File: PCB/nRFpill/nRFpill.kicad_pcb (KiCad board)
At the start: 2 copper layers, 90.7 x 52.7 mm, 138 parts, among them J1 USB_C_Receptacle_USB2.0, J10 , J11 USB_C_Receptacle_USB2.0, J12 , J13 , J14 , J15 , J16 USB_C_Receptacle_USB2.0, J17 , J18 , J19 , J2 , J20 , J3 , J4 , J5 , J6 USB_C_Receptacle_USB2.0, J7 , J8 , J9 , Q1 AO3407, Q2 AO3407, Q3 AO3407, Q4 AO3407, Q5 AO3407, Q6 AO3407, Q7 AO3407, Q8 AO3407, SW1 RST, SW2 DFU, SW3 RST, SW4 DFU, SW5 RST, SW6 DFU, SW7 RST, SW8 DFU, U1 MIC5219-3.3YM5, U10 USBLC6-2SC6, U11 TP4054, U12 MS88FS3, U13 MIC5219-3.3YM5, U14 USBLC6-2SC6, U15 TP4054, U16 MS88FS3, U2 USBLC6-2SC6, U3 TP4054, U4 MIC5219-3.3YM5, U5 MS88FS3, U6 USBLC6-2SC6, U7 TP4054, U8 MS88FS3, U9 MIC5219-3.3YM5

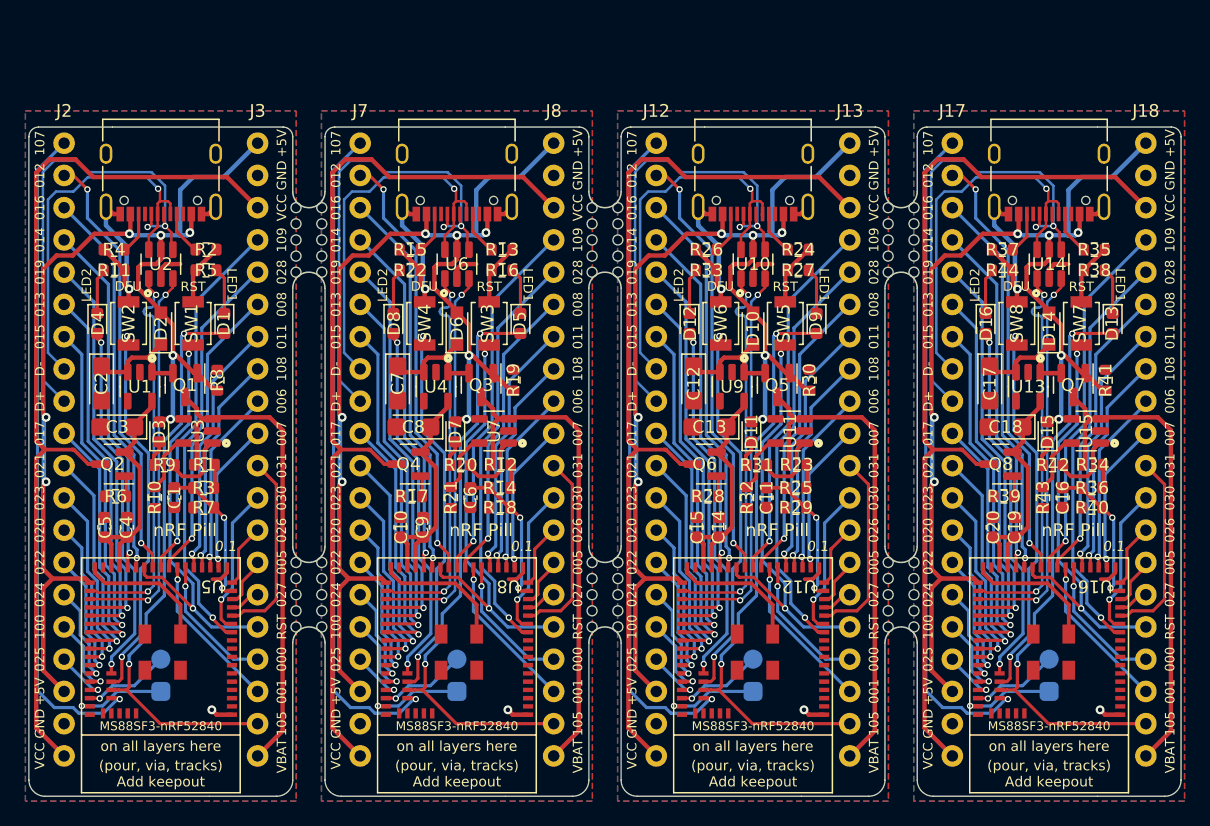
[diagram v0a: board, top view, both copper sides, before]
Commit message: update file
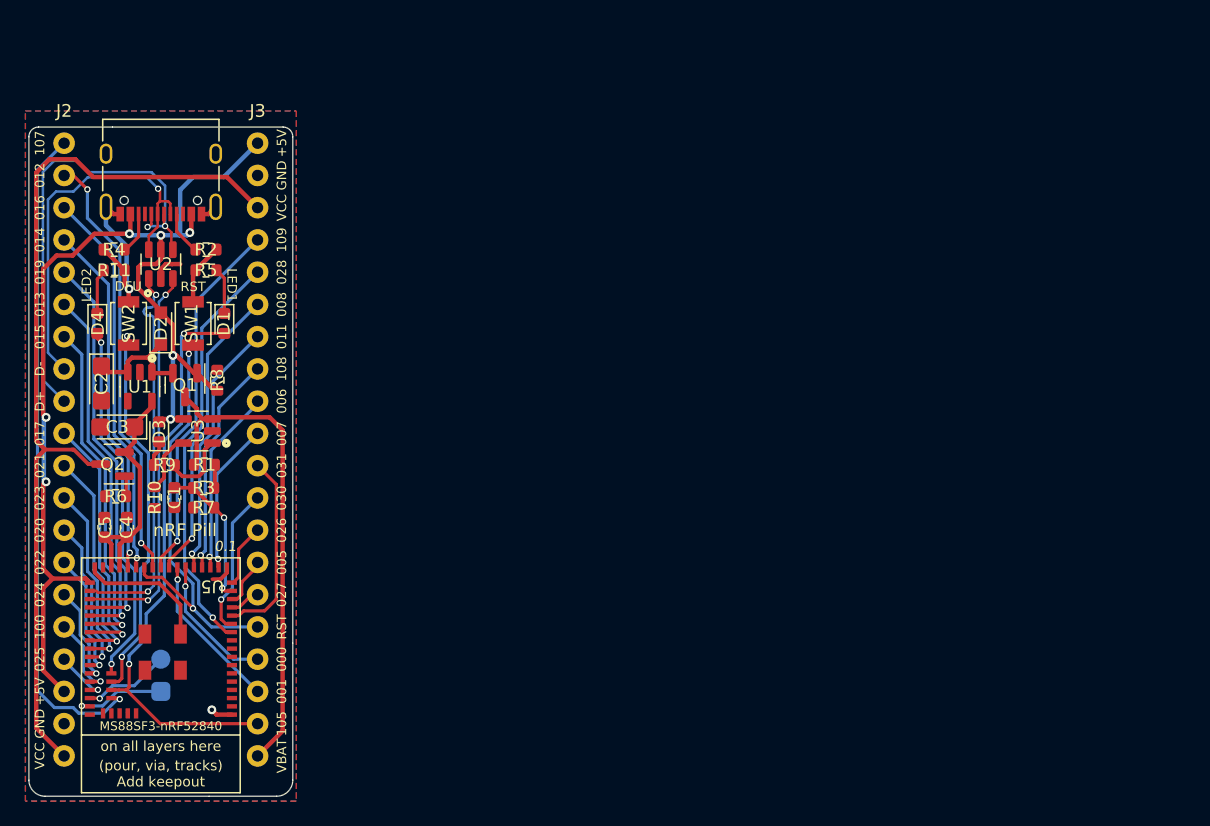
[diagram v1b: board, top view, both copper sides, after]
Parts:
- removed C10, C15, C20: 0.1uF, Capacitor_SMD:C_0603_1608Metric
- removed C11, C16, C6: 100nF, Capacitor_SMD:C_0603_1608Metric
- removed C12, C13, C17, C18, C7, C8: 10uF, Capacitor_Tantalum_SMD:CP_EIA-3216-12_Kemet-S
- removed C14, C19, C9: 10uF, Capacitor_SMD:C_0603_1608Metric
- removed D10, D14, D6: 1N5819, Diode_SMD:D_SOD-323_HandSoldering
- removed D11, D12, D13, D15, D16, D5, D7, D8, D9: BLUE, LED_SMD:LED_0603_1608Metric
- removed J10, J15, J20: , TestPoint:TestPoint_Pad_D1.5mm
- removed J11, J16, J6: USB_C_Receptacle_USB2.0, kien242:USB-C-16pin-hight
- removed J12, J13, J17, J18, J7, J8: , Library:PinHeader_1x20_P2.54mm_Vertical
- removed J14, J19, J9: , TestPoint:TestPoint_Pad_1.5x1.5mm
- removed Q3, Q4, Q5, Q6, Q7, Q8: AO3407, Package_TO_SOT_SMD:SOT-23
- removed R12, R14, R17, R23, R25, R28, R34, R36, R39: 2M, Resistor_SMD:R_0603_1608Metric
- removed R13, R15, R24, R26, R35, R37: 5.1k, Resistor_SMD:R_0603_1608Metric
- removed R16, R20, R22, R27, R31, R33, R38, R42, R44: 1K, Resistor_SMD:R_0603_1608Metric
- removed R18, R29, R40: 10M, Resistor_SMD:R_0603_1608Metric
- removed R19, R30, R41: 100K, Resistor_SMD:R_0603_1608Metric
- removed R21, R32, R43: RPROG, Resistor_SMD:R_0603_1608Metric
- removed REF** (x6): breakaway-mousebites, kien242:breakaway-mousebites
- removed SW3, SW5, SW7: RST, Button_Switch_SMD:SW_SPST_B3U-1000P
- removed SW4, SW6, SW8: DFU, Button_Switch_SMD:SW_SPST_B3U-1000P
- removed U10, U14, U6: USBLC6-2SC6, Library:SOT-23-6
- removed U11, U15, U7: TP4054, Library:SOT-23-5
- removed U12, U16, U8: MS88FS3, kien242:MS88SF3-nRF52840
- removed U13, U4, U9: MIC5219-3.3YM5, Library:SOT-23-5
- C1: value 100nF -> 10nF
- R10: value RPROG -> 2k
- R6: value 2M -> 100K
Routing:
- net +5V: track 355.7 -> 88.9 mm, vias 28 -> 7
- net VCC: track 286.9 -> 71.7 mm
- net 1.07: track 209.5 -> 52.4 mm, vias 4 -> 1
- net LED_1: track 183.0 -> 45.7 mm, vias 8 -> 2
- net VBAT: track 157.8 -> 39.5 mm
- net DP+: track 153.9 -> 38.5 mm, vias 8 -> 2
- net GND: track 145.1 -> 36.3 mm, vias 8 -> 2
- net 0.12: track 136.8 -> 34.2 mm, vias 8 -> 2
- net RST: track 133.8 -> 33.4 mm, vias 8 -> 2
- net 0.28: track 130.2 -> 32.5 mm, vias 4 -> 1
- net 0.19: track 126.0 -> 31.5 mm, vias 4 -> 1
- net D-: track 123.4 -> 30.8 mm, vias 8 -> 2
- net D+: track 123.3 -> 30.8 mm, vias 8 -> 2
- net 0.16: track 123.0 -> 30.7 mm, vias 4 -> 1
- net DP-: track 122.6 -> 30.7 mm, vias 4 -> 1
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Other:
- board size 90.7 x 52.7 mm -> 20.8 x 52.7 mm

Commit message: cap nhat
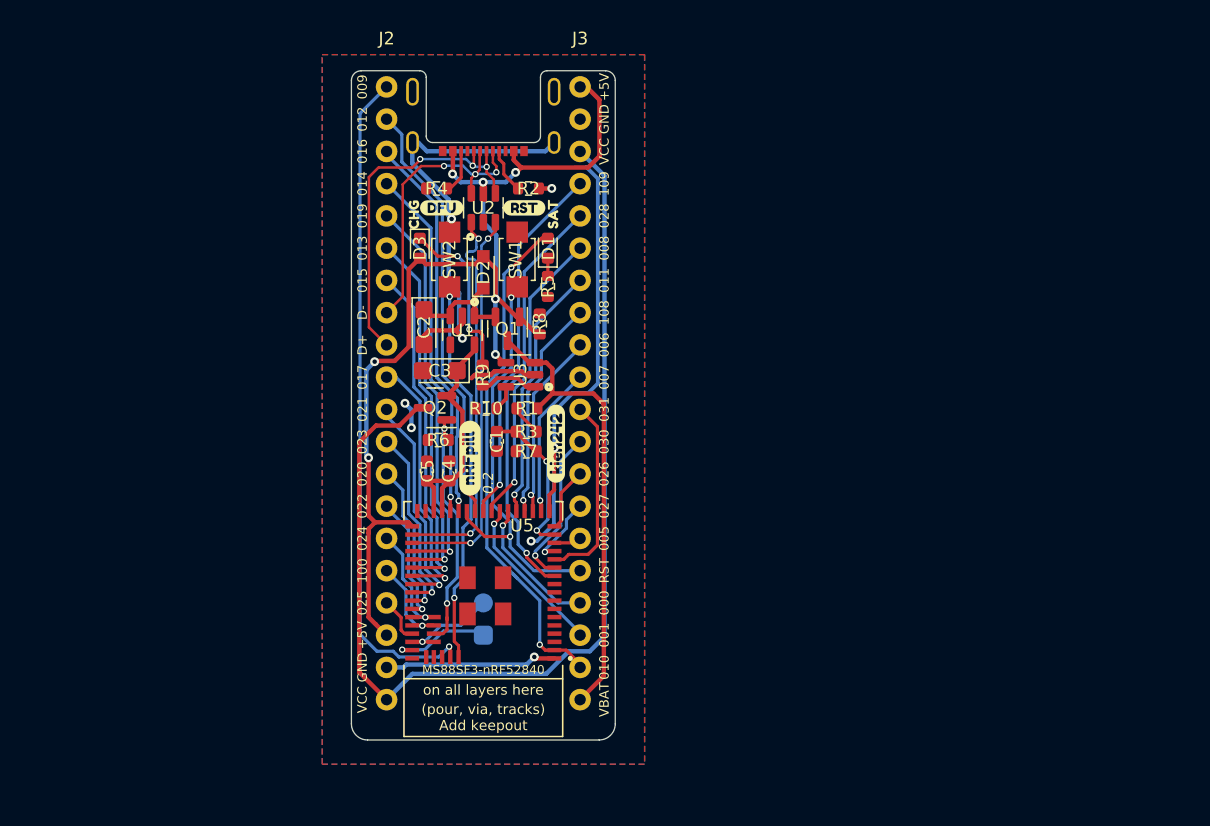
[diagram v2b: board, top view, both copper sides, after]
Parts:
- removed D4: BLUE, LED_SMD:LED_0603_1608Metric
- removed R11: 1K, Resistor_SMD:R_0603_1608Metric
- added kibuzzard-62FEE358: G***, kibuzzard-62FEE358, B.Cu at (76.2, 73.8)
- added kibuzzard-62FEE3AB: G***, kibuzzard-62FEE3AB, B.Cu at (78.0, 71.5)
- added kibuzzard-6303CF12: G***, kibuzzard-6303CF12, F.Cu at (75.2, 54.6)
- added kibuzzard-6303CF50: G***, kibuzzard-6303CF50, F.Cu at (81.9, 53.5)
- added kibuzzard-6303CFD4: G***, kibuzzard-6303CFD4, F.Cu at (70.7, 35.5)
- added kibuzzard-6303D094: G***, kibuzzard-6303D094, F.Cu at (81.7, 35.4)
- added kibuzzard-63049CD9: G***, kibuzzard-63049CD9, F.Cu at (72.9, 34.9)
- added kibuzzard-63049CF8: G***, kibuzzard-63049CF8, F.Cu at (79.4, 34.9)
- C1: value 10nF -> 100nF
- C5: value 0.1uF -> 100nF
- J1: footprint kien242:USB-C-16pin-hight -> kien242:USB-C-Low
- R10: value 2k -> 2.3k
- R6: value 100K -> 100k
- U5: footprint kien242:MS88SF3-nRF52840 -> kien242:MODULE_MS88SF3
- moved R10 27.0 mm to (76.4, 50.7), turned to 180 degrees
- moved R5 27.0 mm to (81.3, 41.1), turned to 90 degrees
- moved D1 26.2 mm to (81.3, 38.1), turned to 90 degrees
- moved R9 26.1 mm to (76.2, 48.1), turned to -90 degrees
- moved SW1 26.0 mm to (78.9, 39.0)
- moved R2 25.9 mm to (79.8, 33.4)
- moved R4 25.9 mm to (72.5, 33.4)
- moved C1 25.8 mm to (77.3, 53.3)
- moved D2 25.8 mm to (76.2, 40.0)
- moved J4 25.8 mm to (76.2, 68.6)
- moved J5 25.8 mm to (76.2, 66.1)
- moved Q1 25.8 mm to (78.1, 44.5)
- moved R1 25.8 mm to (79.6, 50.7), turned to 180 degrees
- moved R6 25.8 mm to (72.6, 53.2)
- moved U1 25.8 mm to (74.5, 44.6)
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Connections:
- J2 pad 1: 1.07 -> 009
- J3 pad 14: 0.05 -> 0.27
- J3 pad 15: 0.27 -> 0.05
- U5 pad 2: unconnected-(U5-Pad2) -> LED_1
- U5 pad 55: unconnected-(U5-Pad55) -> 009
- U5 pad 56: unconnected-(U5-Pad56) -> DFU
- U5 pad 57: 1.07 -> SWDIO
- U5 pad 58: LED_1 -> POWER_PIN
- U5 pad 59: DFU -> 1.00
- U5 pad 60: LED_2 -> 0.24
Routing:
- net GND: track 36.3 -> 96.4 mm, vias 2 -> 8
- net 009: track 0.00 -> 53.0 mm, vias 0 -> 1
- net 1.07: track 52.4 -> 0.00 mm, vias 1 -> 0
- net LED_2: track 28.8 -> 0.00 mm, vias 2 -> 0
- net POWER_PIN: track 1.59 -> 19.8 mm, vias 0 -> 2
- net VCC: track 71.7 -> 85.9 mm
- net Net-(D3-Pad1): track 2.00 -> 13.3 mm, vias 0 -> 2
- net DP+: track 38.5 -> 28.8 mm, vias 2 -> 3
- net DP-: track 30.7 -> 24.4 mm, vias 1 -> 3
- net LED_1: track 45.7 -> 40.6 mm
- net Net-(D4-Pad1): track 3.29 -> 0.00 mm
- net 0.27: track 2.43 -> 5.54 mm, vias 0 -> 1
- net Net-(R10-Pad1): track 4.71 -> 2.02 mm
- net VBAT: track 39.5 -> 36.8 mm
- net Net-(D1-Pad1): track 3.66 -> 1.42 mm
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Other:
- outline, holes or cut-outs redrawn
- board text added: "0.2"
- board text added: "009"
- board text added: "010"
- board text added: "Bình Ngô đại cáo - 1428 Nguyễn Trãi"
- board text added: "v0.2"
- board text added: "Đem đại nghĩa để thắng hung tàn, Lấy chí nhân để thay cường bạo."
- board text removed: "0.1"
- board text removed: "105"
- board text removed: "107"
- board text removed: "DFU"
- board text removed: "LED1"
- board text removed: "LED2"
- board text removed: "nRF Pill"
- board text removed: "nRFPill"
